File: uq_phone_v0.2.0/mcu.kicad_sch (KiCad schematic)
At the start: 34 parts, among them J6 Conn_ARM_SWD_TagConnect_TC2030, J7 559092474, J9 559092474, Q1 MMBT3904LP-7, Q2 MMBT3904LP-7, U16 TXB0108YZPR2, U5 TCA9509MRVHR, U6 STM32H733VGHx, U7 TXB0108YZPR2

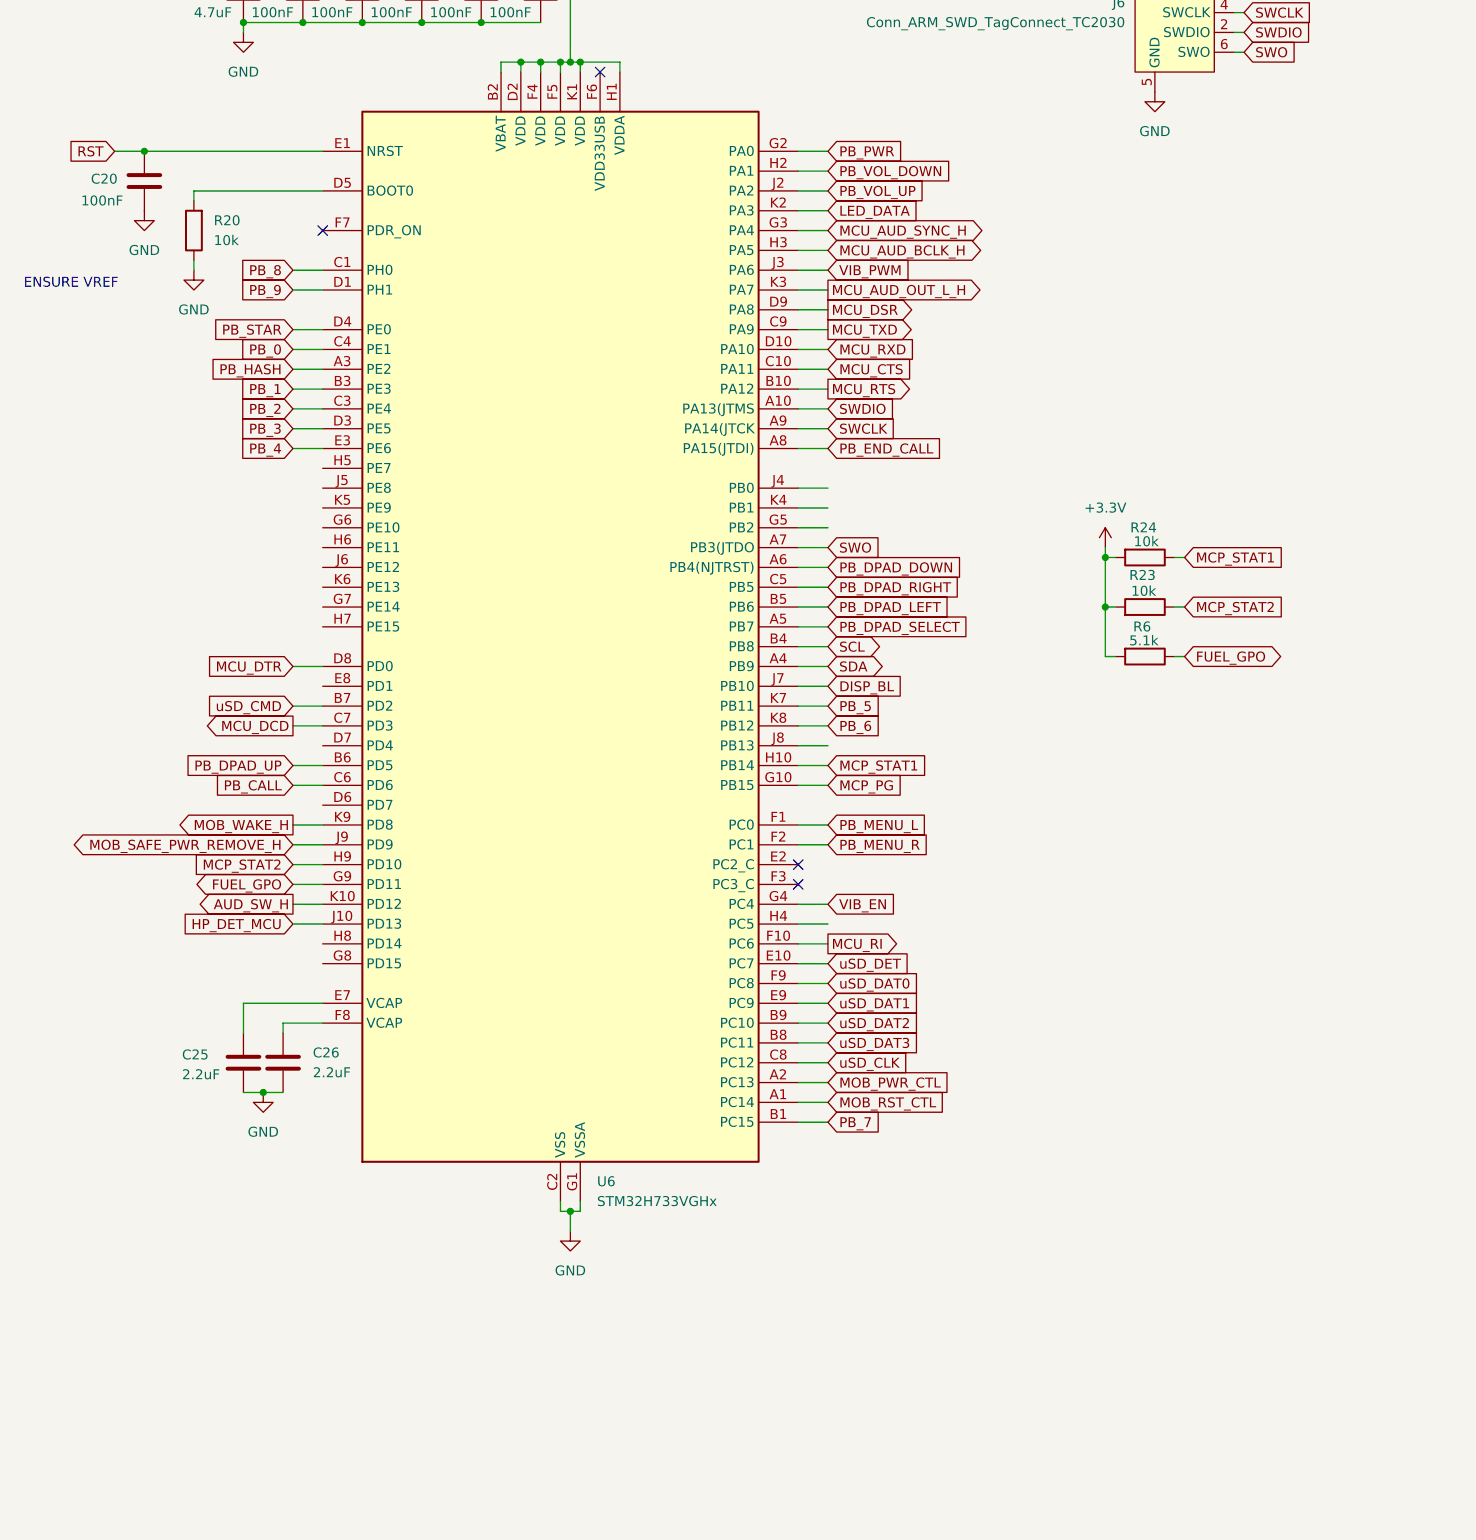
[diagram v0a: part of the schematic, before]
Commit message: More routing and moving cellular to new project
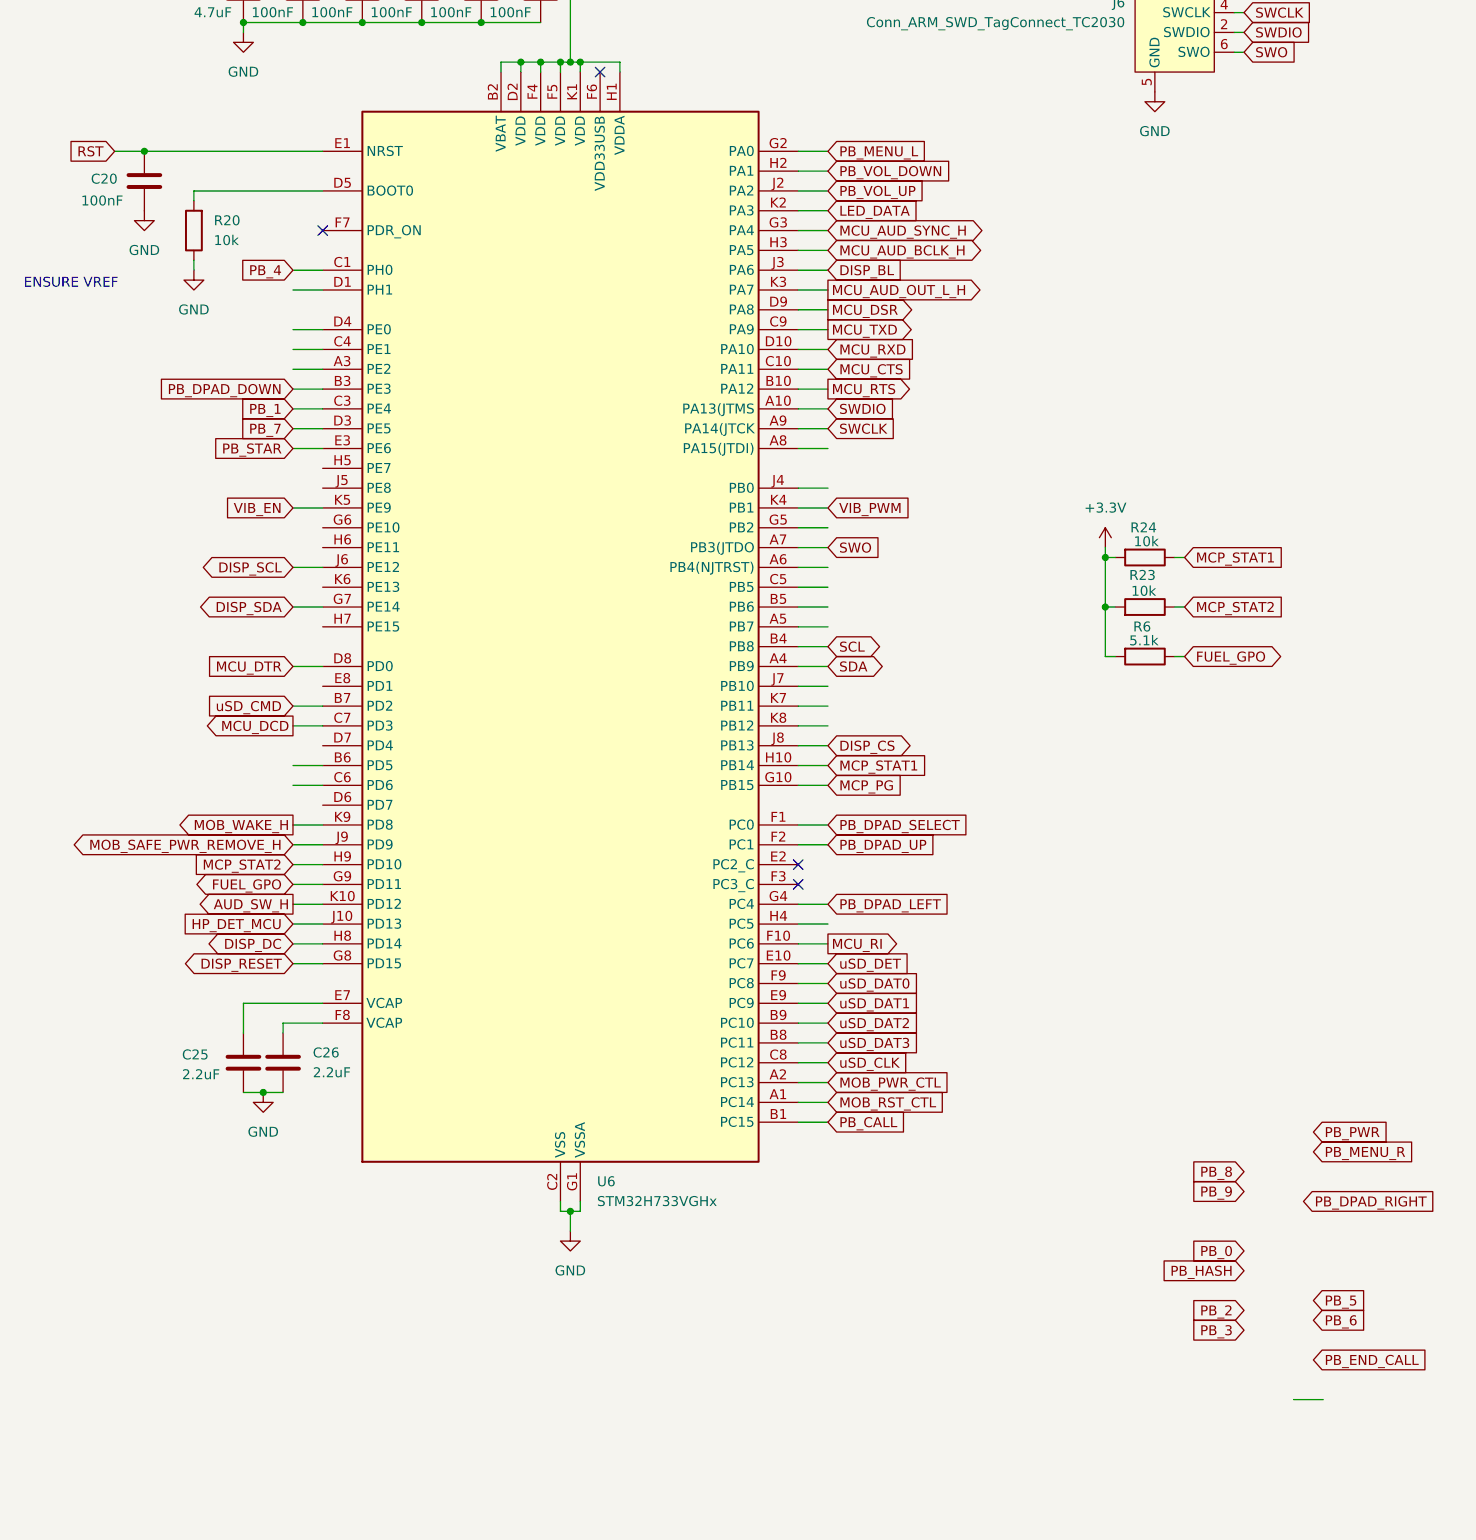
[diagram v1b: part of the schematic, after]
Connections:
- net DISP_BL: now also U6.J3 (PA6); no longer U6.J7 (PB10)
- net PB_0: no longer U6.C4 (PE1)
- net PB_1: now also U6.C3 (PE4); no longer U6.B3 (PE3)
- net PB_2: no longer U6.C3 (PE4)
- net PB_3: no longer U6.D3 (PE5)
- net PB_4: now also U6.C1 (PH0); no longer U6.E3 (PE6)
- net PB_5: no longer U6.K7 (PB11)
- net PB_6: no longer U6.K8 (PB12)
- net PB_7: now also U6.D3 (PE5); no longer U6.B1 (PC15)
- net PB_8: no longer U6.C1 (PH0)
- net PB_9: no longer U6.D1 (PH1)
- net PB_CALL: now also U6.B1 (PC15); no longer U6.C6 (PD6)
- net PB_DPAD_DOWN: now also U6.B3 (PE3); no longer U6.A6 (PB4(NJTRST))
- net PB_DPAD_LEFT: now also U6.G4 (PC4); no longer U6.B5 (PB6)
- net PB_DPAD_RIGHT: no longer U6.C5 (PB5)
- net PB_DPAD_SELECT: now also U6.F1 (PC0); no longer U6.A5 (PB7)
- net PB_DPAD_UP: now also U6.F2 (PC1); no longer U6.B6 (PD5)
- net PB_END_CALL: no longer U6.A8 (PA15(JTDI))
- net PB_HASH: no longer U6.A3 (PE2)
- net PB_MENU_L: now also U6.G2 (PA0); no longer U6.F1 (PC0)
- net PB_MENU_R: no longer U6.F2 (PC1)
- net PB_PWR: no longer U6.G2 (PA0)
- net PB_STAR: now also U6.E3 (PE6); no longer U6.D4 (PE0)
- net VIB_EN: now also U6.K5 (PE9); no longer U6.G4 (PC4)
- net VIB_PWM: now also U6.K4 (PB1); no longer U6.J3 (PA6)
- net DISP_SDA: now reaches U6.G7 (PE14)
- net DISP_RESET: now reaches U6.G8 (PD15)
- net DISP_DC: now reaches U6.H8 (PD14)
- net DISP_SCL: now reaches U6.J6 (PE12)
- net DISP_CS: now reaches U6.J8 (PB13)

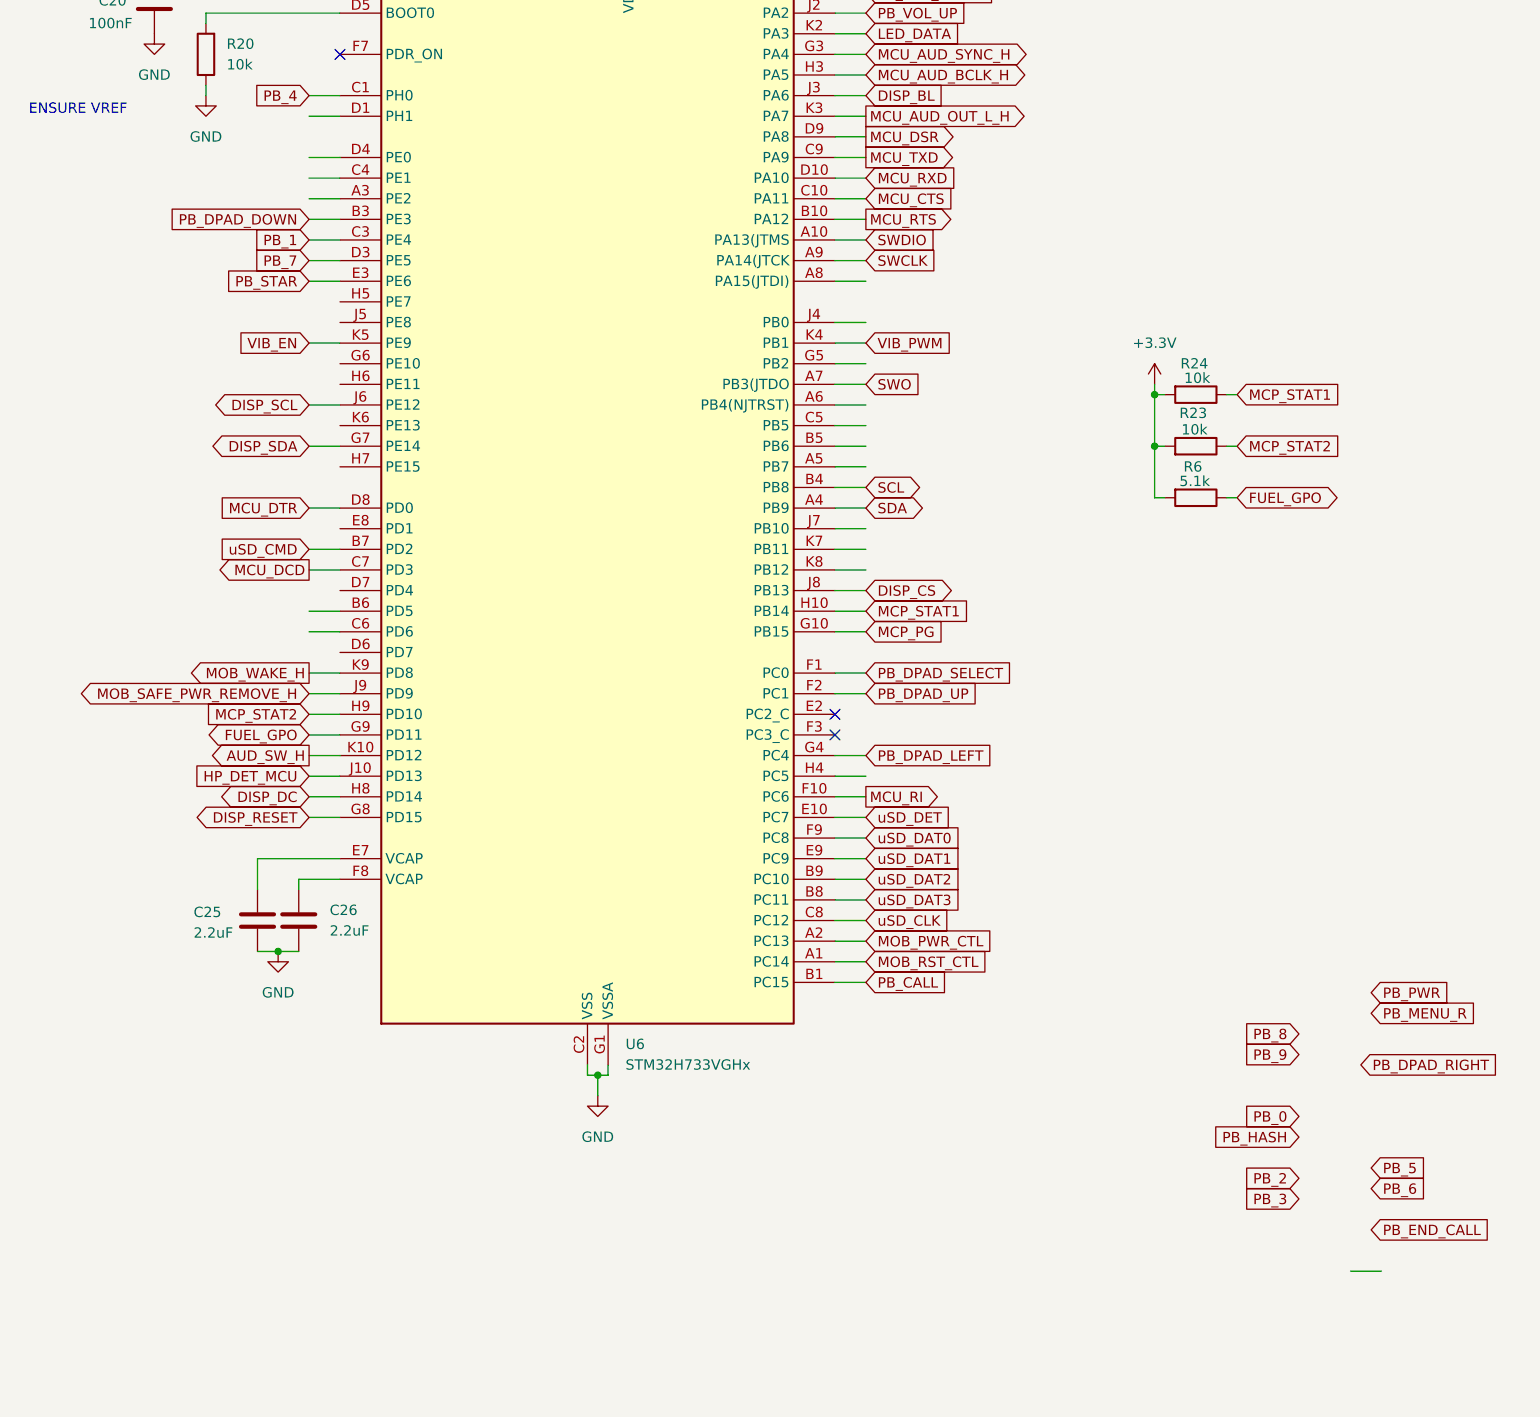
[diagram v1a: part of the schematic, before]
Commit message: Most routing complete
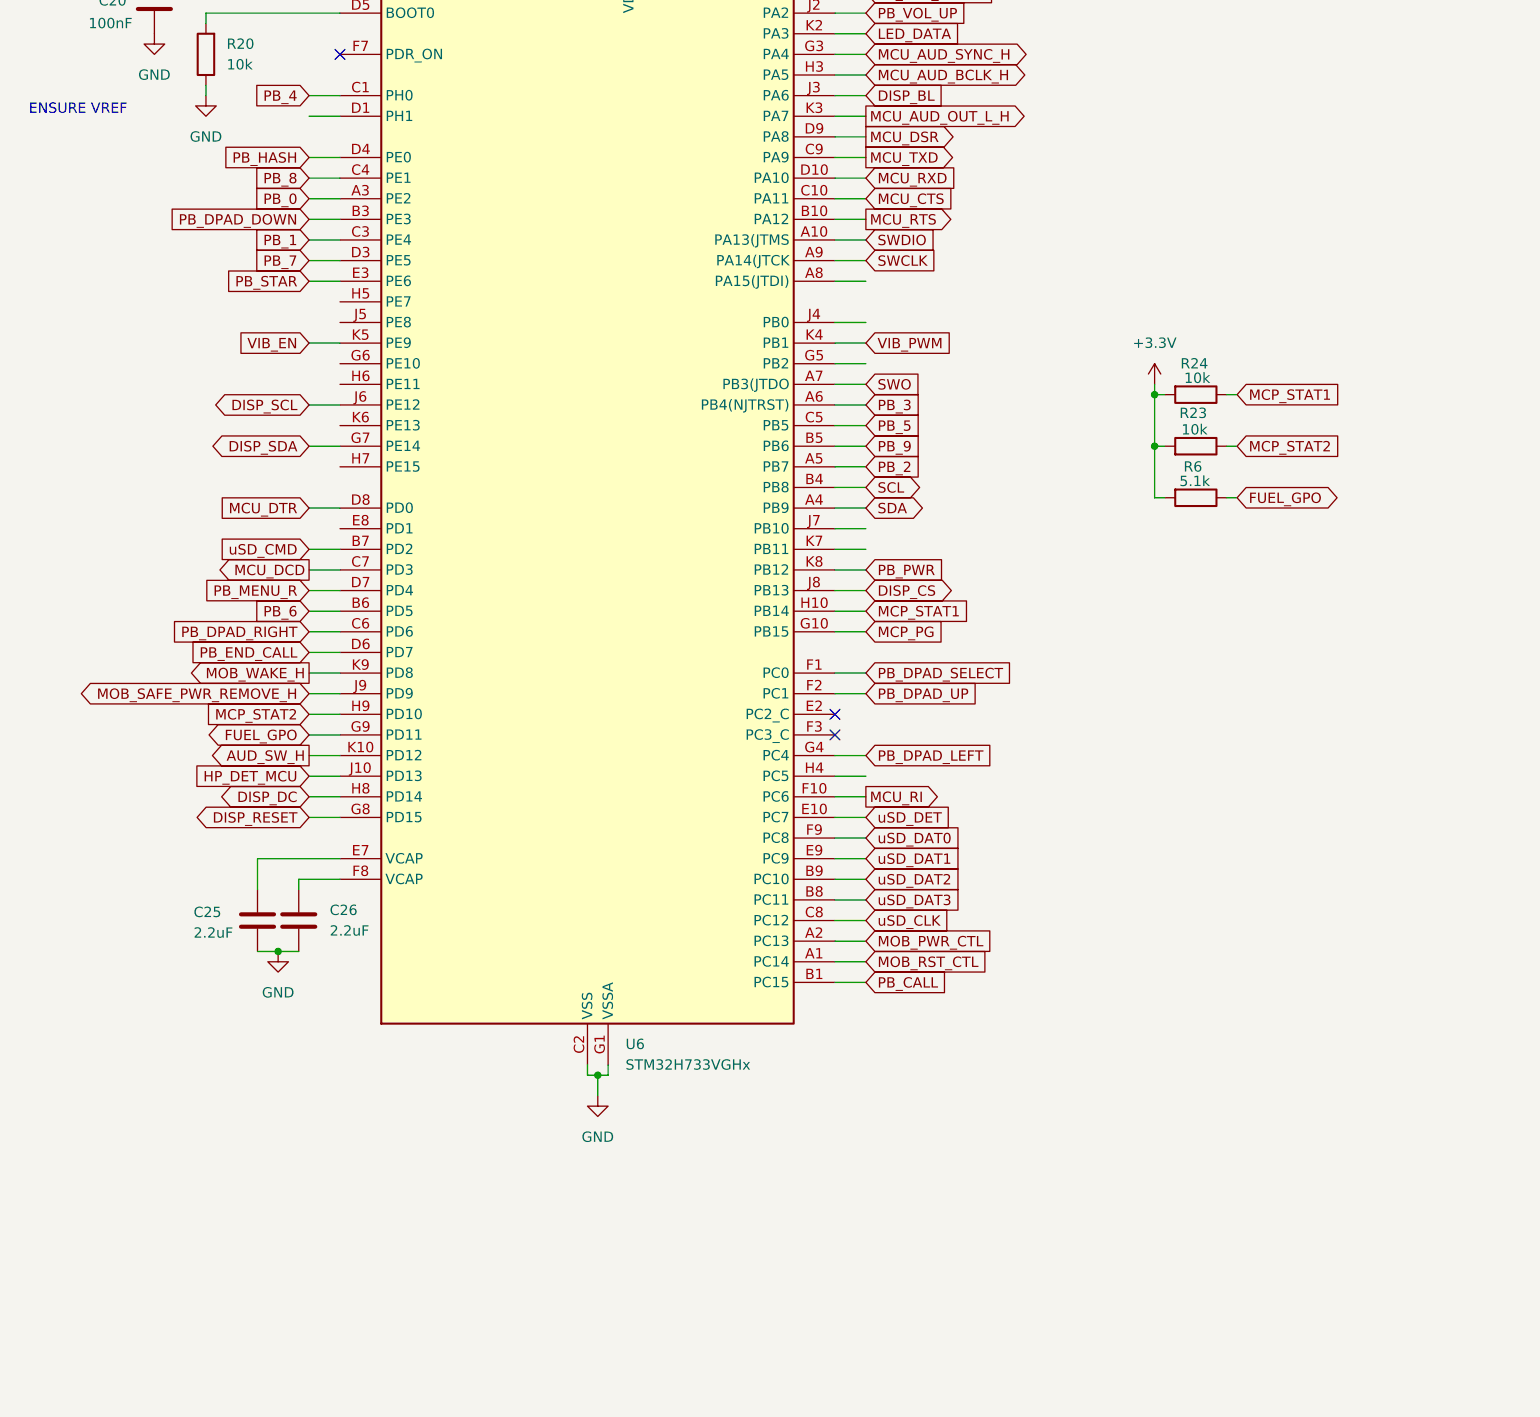
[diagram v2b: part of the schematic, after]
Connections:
- net PB_0: now also U6.A3 (PE2)
- net PB_2: now also U6.A5 (PB7)
- net PB_3: now also U6.A6 (PB4(NJTRST))
- net PB_5: now also U6.C5 (PB5)
- net PB_6: now also U6.B6 (PD5)
- net PB_8: now also U6.C4 (PE1)
- net PB_9: now also U6.B5 (PB6)
- net PB_DPAD_RIGHT: now also U6.C6 (PD6)
- net PB_END_CALL: now also U6.D6 (PD7)
- net PB_HASH: now also U6.D4 (PE0)
- net PB_MENU_R: now also U6.D7 (PD4)
- net PB_PWR: now also U6.K8 (PB12)
